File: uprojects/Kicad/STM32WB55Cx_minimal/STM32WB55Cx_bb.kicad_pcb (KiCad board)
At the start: 2 copper layers, 17.8 x 38.1 mm, 33 parts, among them J1 Prog, J2 USB, J3 GPIO1, J4 GPIO2, U1 STM32WB55Cx, U2 LDFM, Y1 LSE, Y2 32MHz

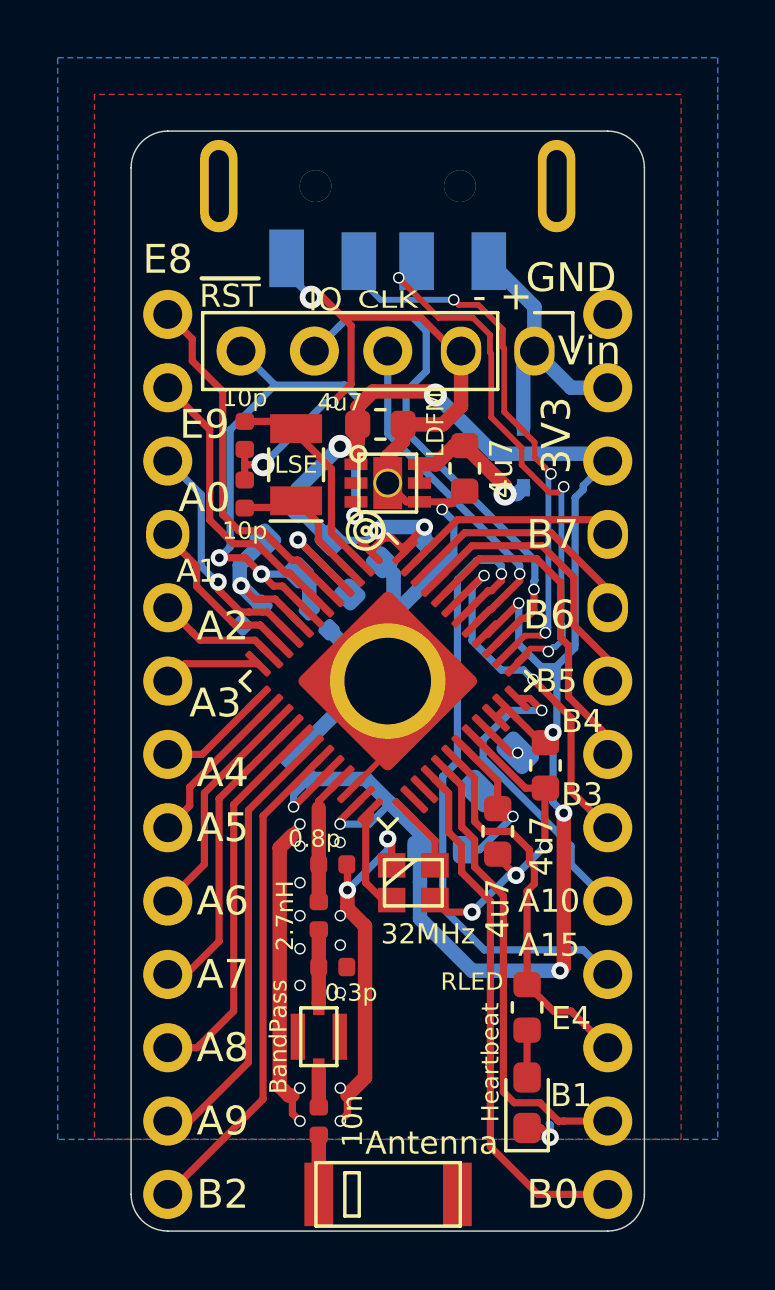
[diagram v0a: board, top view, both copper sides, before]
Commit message: 23 Mar 2025 Dorm
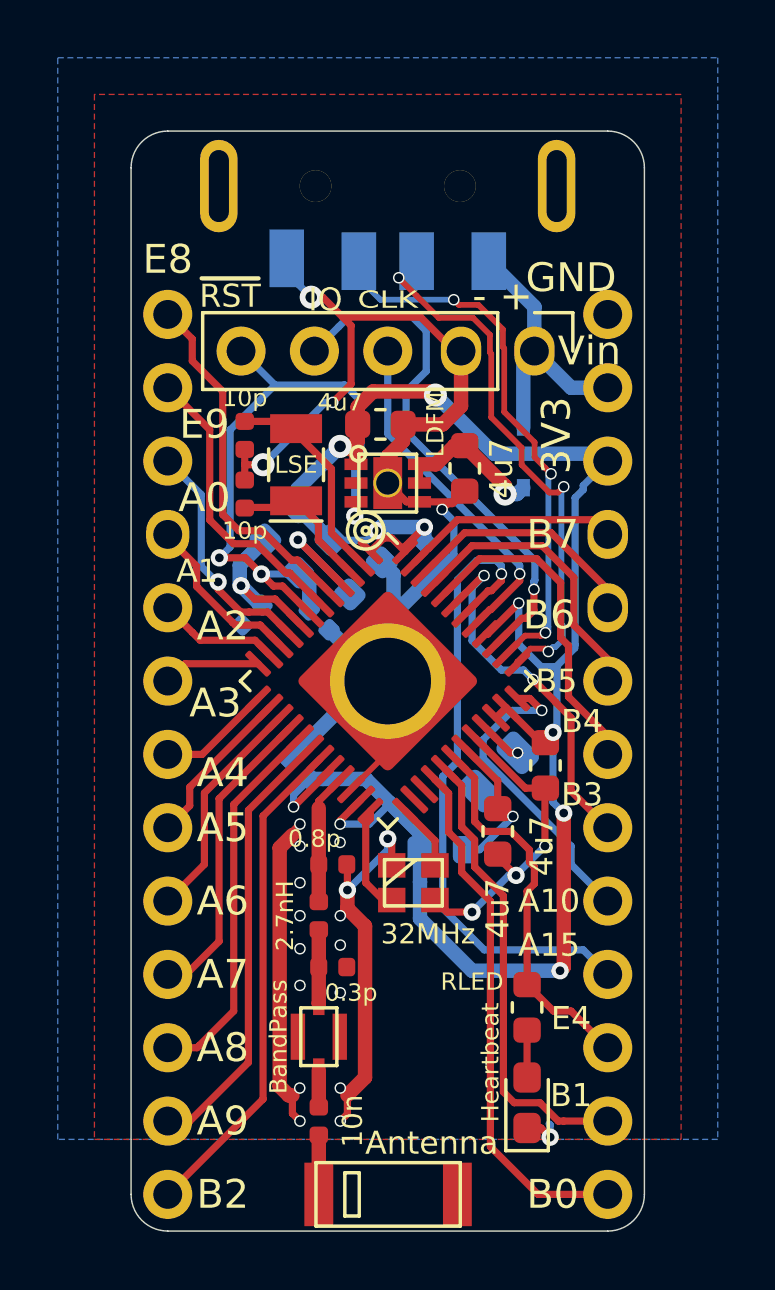
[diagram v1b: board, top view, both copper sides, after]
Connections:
- net ~RST renamed ~{RST}
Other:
- net class Default removed
- board text added: "~{RST}"
- board text removed: "~RST"
